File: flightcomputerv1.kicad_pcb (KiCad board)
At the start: 4 copper layers, 100 x 65.5 mm, 54 parts, among them IC1 MMC5983MA, J1 Screw_Terminal_01x02, J2 Screw_Terminal_01x02, J5 Conn_01x02, J6 Conn_01x24, J7 Conn_01x24, J8 Conn_Coaxial, J9 Conn_Coaxial, M1 Motor_Servo, M2 Motor_Servo, Q1 SI4925DDY-T1-GE3, Q2 MMBT3904, Q3 MMBT3904, U1 Teensy4.1, U2 MS5607-02BA, U3 BMI088, U4 MIC29302AWD, U5 MAX-M10S, U6 RFM95W-915S2, U7 LD1117S50TR_SOT223

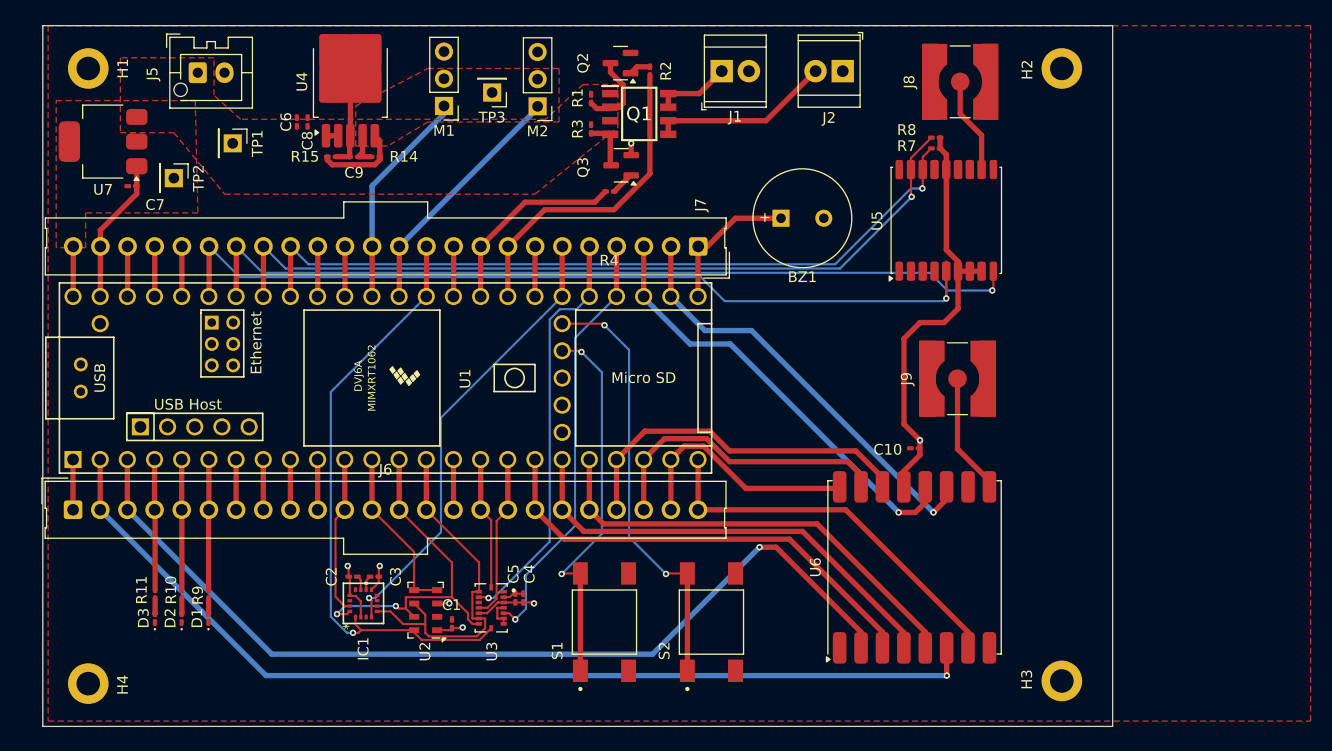
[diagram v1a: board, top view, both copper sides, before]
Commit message: 2025 FINAL
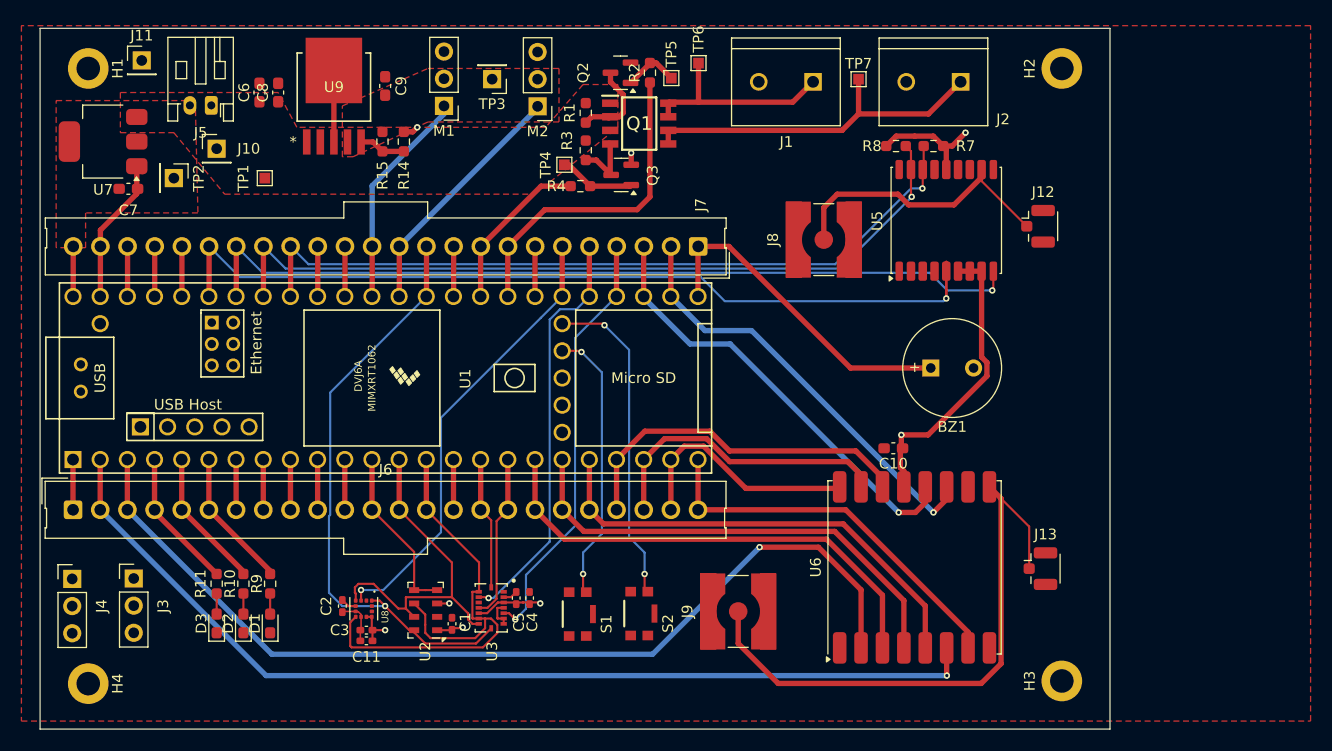
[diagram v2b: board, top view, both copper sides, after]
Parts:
- removed IC1: MMC5983MA, HPRfootprints:MMC5983MA_MEM
- removed U4: MIC29302AWD, Package_TO_SOT_SMD:TO-252-5_TabPin3
- added C11: 100nF, Capacitor_SMD:C_0402_1005Metric_Pad0.74x0.62mm_HandSolder, F.Cu at (79.8, 117.2)
- added G***: LOGO, HPRfootprints:HPRLOGOSILK, B.Cu at (101.5, 93.5)
- added J10: Conn_01x01, Connector_PinHeader_2.54mm:PinHeader_1x01_P2.54mm_Vertical, F.Cu at (65.8, 71.2)
- added J11: Conn_01x01, Connector_PinHeader_2.54mm:PinHeader_1x01_P2.54mm_Vertical, F.Cu at (58.8, 63.0)
- added J12: Conn_Coaxial, Connector_Coaxial:U.FL_Hirose_U.FL-R-SMT-1_Vertical, F.Cu at (142.5, 78.5)
- added J13: Conn_Coaxial, Connector_Coaxial:U.FL_Hirose_U.FL-R-SMT-1_Vertical, F.Cu at (142.8, 110.5)
- added J3: Conn_01x03, Connector_PinHeader_2.54mm:PinHeader_1x03_P2.54mm_Vertical, F.Cu at (58.0, 111.4)
- added J4: Conn_01x03, Connector_PinHeader_2.54mm:PinHeader_1x03_P2.54mm_Vertical, F.Cu at (52.2, 111.5)
- added TP4: TestPoint, TestPoint:TestPoint_Pad_1.0x1.0mm, F.Cu at (98.2, 72.8)
- added TP5: TestPoint, TestPoint:TestPoint_Pad_1.0x1.0mm, F.Cu at (108.2, 64.7)
- added TP6: TestPoint, TestPoint:TestPoint_Pad_1.0x1.0mm, F.Cu at (110.8, 63.2)
- added TP7: TestPoint, TestPoint:TestPoint_Pad_1.0x1.0mm, F.Cu at (125.8, 64.8)
- added U8: LIS2MDLTR, HPRfootprints:PQFN50P200X200X70-12N, F.Cu at (79.5, 114.2)
- added U9: MIC29302AWD-TR, HPRfootprints:TO-252-5_MCH, F.Cu at (76.7, 65.5)
- C1, C3, C4, C5: footprint Capacitor_SMD:C_0201_0603Metric_Pad0.64x0.40mm_HandSolder -> Capacitor_SMD:C_0402_1005Metric_Pad0.74x0.62mm_HandSolder
- C10, C6, C7, C8, C9: footprint Capacitor_SMD:C_0201_0603Metric_Pad0.64x0.40mm_HandSolder -> Capacitor_SMD:C_0603_1608Metric_Pad1.08x0.95mm_HandSolder
- C2: value 1uF -> 220nF; footprint Capacitor_SMD:C_0201_0603Metric_Pad0.64x0.40mm_HandSolder -> Capacitor_SMD:C_0402_1005Metric_Pad0.74x0.62mm_HandSolder
- D1, D2, D3: footprint LED_SMD:LED_0201_0603Metric_Pad0.64x0.40mm_HandSolder -> LED_SMD:LED_0603_1608Metric_Pad1.05x0.95mm_HandSolder
- J1, J2: value Screw_Terminal_01x02 -> 282837-2; footprint TerminalBlock_TE-Connectivity:TerminalBlock_TE_282834-2_1x02_P2.54mm_Horizontal -> HPRfootprints:TE_282837-2
- J5: footprint Connector_JST:JST_XA_B02B-XASK-1-A_1x02_P2.50mm_Vertical -> Connector_JST:JST_PH_S2B-PH-K_1x02_P2.00mm_Horizontal
- R1, R10, R11, R14, R15, R2, R3, R4, R7, R8, R9: footprint Resistor_SMD:R_0201_0603Metric_Pad0.64x0.40mm_HandSolder -> Resistor_SMD:R_0603_1608Metric_Pad0.98x0.95mm_HandSolder
- S1, S2: value TS04-66-70-BK-160-SMT -> KMR221GLFS; footprint HPRfootprints:SW_TS04-66-70-BK-160-SMT -> HPRfootprints:SW_KMR221GLFS
- TP1: footprint Connector_PinHeader_2.54mm:PinHeader_1x01_P2.54mm_Vertical -> TestPoint:TestPoint_Pad_1.0x1.0mm
- moved J9 29.9 mm to (114.5, 114.5)
- moved BZ1 19.8 mm to (132.5, 91.8)
- moved J8 19.5 mm to (122.5, 79.8)
- moved J2 8.54 mm to (132.8, 65.0)
- moved C9 7.22 mm to (81.5, 65.4), turned to 90 degrees
- moved S2 6.80 mm to (105.2, 114.7), turned to -90 degrees
- moved J1 6.08 mm to (119.0, 65.0), turned to 180 degrees
- moved R10 5.83 mm to (68.2, 111.9)
- moved R11 5.83 mm to (65.8, 111.9)
- moved R9 5.83 mm to (70.8, 111.9)
- moved D2 5.79 mm to (68.2, 115.6)
- moved D3 5.79 mm to (65.8, 115.6)
- moved D1 5.79 mm to (70.8, 115.6)
- moved C3 5.06 mm to (79.8, 116.2), turned to 180 degrees
- moved R15 4.96 mm to (81.2, 70.6), turned to 90 degrees
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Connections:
- net /mag_int renamed /FREE2
- C2 pad 1: /teensy_3.3v -> Net-(U8-C1)
- C3 pad 1: Net-(IC1-CAP) -> /teensy_3.3v
- J2 pad 1: GND -> Net-(Q1-D2_1)
- J2 pad 2: Net-(J2-Pin_2) -> GND
- Q1 pad 5: Net-(J2-Pin_2) -> Net-(Q1-D2_1)
- Q1 pad 6: Net-(J2-Pin_2) -> Net-(Q1-D2_1)
- R14 pad 2: /ldo_6v -> GND
- R15 pad 2: GND -> /ldo_6v
- S1 pad 3: Net-(U1-PROGRAM) -> (no net)
- S1 pad 4: GND -> (no net)
- S2 pad 3: /teensy_onoff -> (no net)
- S2 pad 4: GND -> (no net)
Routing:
- net Net-(J13-In): track 11.3 -> 56.0 mm
- net Net-(Q1-D2_1): track 0.00 -> 33.7 mm
- net Net-(J12-In): track 9.03 -> 27.5 mm
- net /buzz_pwm: track 13.5 -> 31.1 mm
- net Net-(J2-Pin_2): track 17.0 -> 0.00 mm
- net /SENSE_miso: track 33.8 -> 48.4 mm
- net Net-(Q1-D1_1): track 7.14 -> 19.3 mm
- net /FREE2: track 15.0 -> 4.78 mm
- net /teensy_onoff: track 40.8 -> 30.6 mm
- net Net-(U1-PROGRAM): track 35.8 -> 25.9 mm
- net Net-(Q3-B): track 2.21 -> 7.12 mm
- net Net-(U9-ADJ): track 8.02 -> 4.37 mm
- net Net-(Q2-B): track 2.06 -> 5.55 mm
- net /ldo_6v: track 3.31 -> 0.06 mm
- net /PYRO2: track 18.5 -> 15.4 mm
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- added copper zone on In2.Cu, net /ldo_5v
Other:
- rule pad_to_mask_clearance: 0 -> 0.1
